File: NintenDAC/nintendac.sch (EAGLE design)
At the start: 36 parts, among them IC2 REG1117, U1 STM32F10XRXT6, X1 USB-MICROB

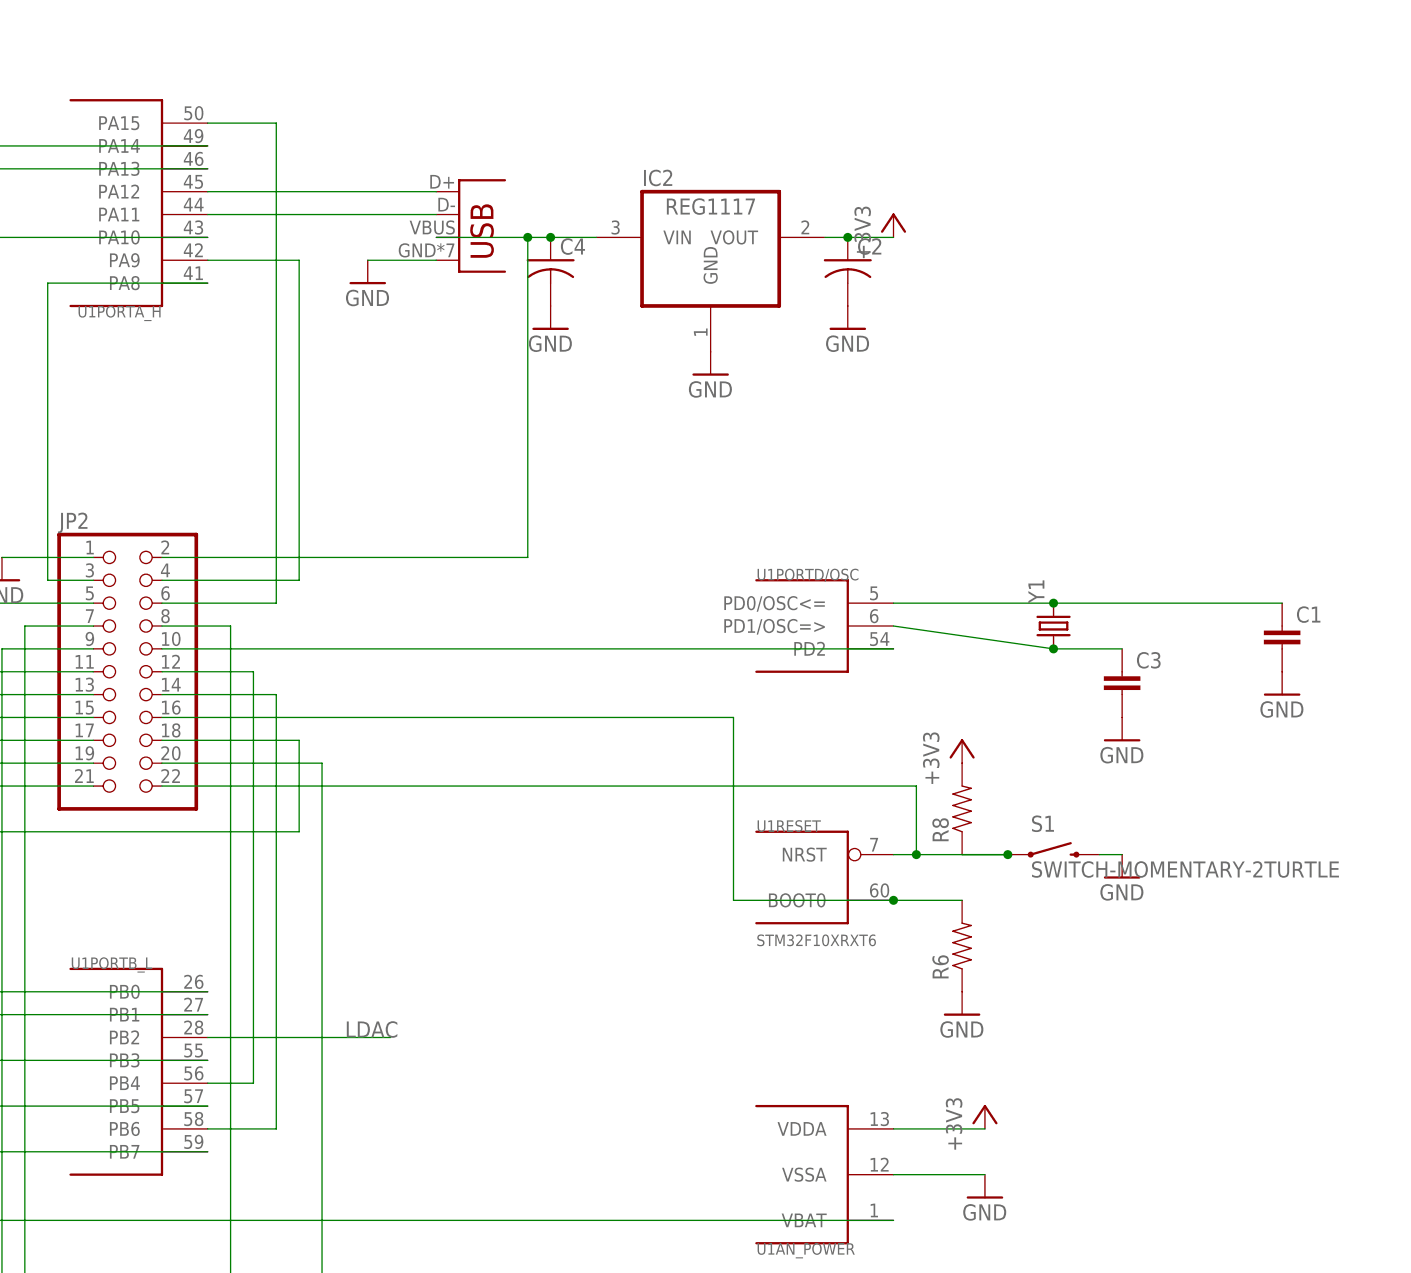
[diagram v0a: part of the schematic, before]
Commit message: board cleanup
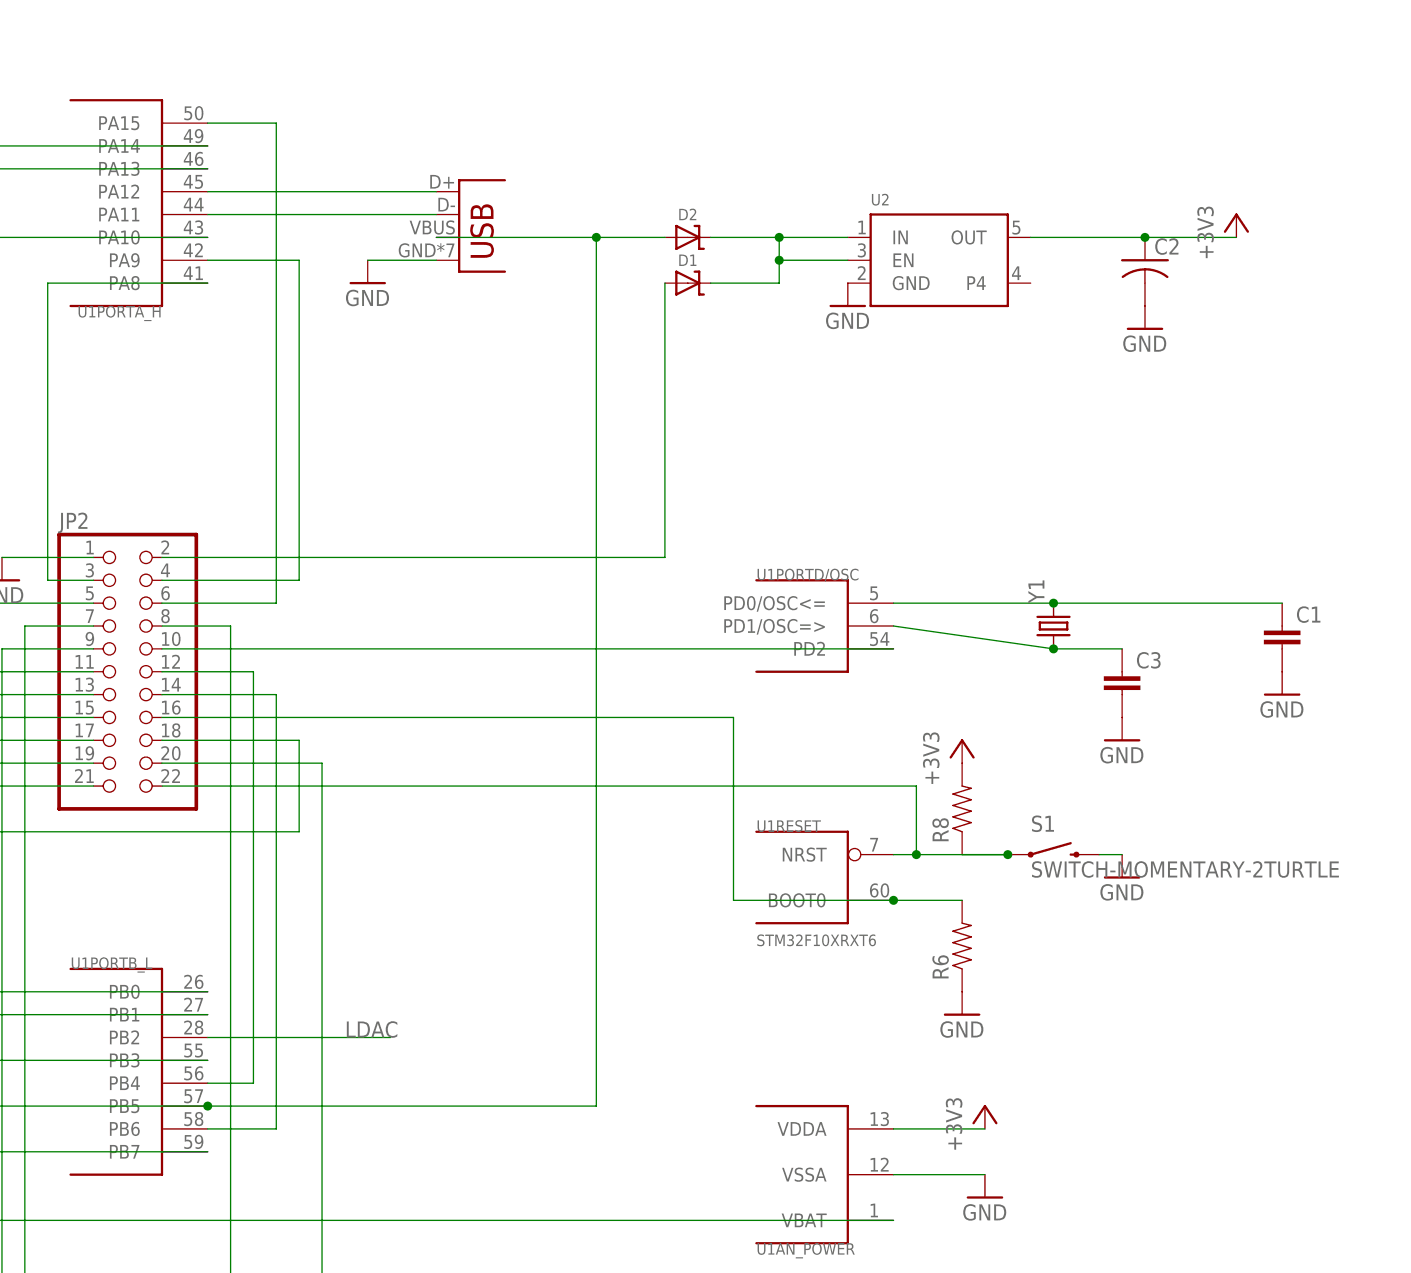
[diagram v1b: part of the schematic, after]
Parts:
- removed C4: (no value), backplane:C-USC1210
- removed IC2: REG1117, backplane:REG1117
- added D1, D2: (no value), nintendac_mini:DIODE-SCHOTTKYSOD-123
- added U2: (no value), nintendac_mini:VREG_SOT23-5
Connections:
- new net N$2: D1.C, D2.C, U2.EN, U2.IN
- net +3V3: now also U2.OUT; no longer IC2.VOUT
- net GND: now also U2.GND; no longer C4.2, IC2.GND
- net N$58: now also D2.A, X1.VBUS
- net N$66: now also D1.A; no longer C4.1, IC2.VIN, X1.VBUS
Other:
- moved on the sheet: C2
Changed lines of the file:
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@@
 <part name="GND1" library="backplane" deviceset="GND" device=""/>
 <part name="R1" library="SparkFun-Passives" deviceset="RESISTOR" device="0805-RES"/>
-<part name="IC2" library="backplane" deviceset="REG1117" device=""/>
 <part name="X1" library="backplane" deviceset="USB" device="-MICROB"/>
 <part name="GND2" library="backplane" deviceset="GND" device=""/>
@@
 <part name="+3V2" library="backplane" deviceset="+3V3" device=""/>
 <part name="GND5" library="backplane" deviceset="GND" device=""/>
-<part name="GND6" library="backplane" deviceset="GND" device=""/>
 <part name="+3V3" library="backplane" deviceset="+3V3" device=""/>
 <part name="S1" library="Adafruit Feather M0 Adalogger" deviceset="SWITCH-MOMENTARY-2" device="TURTLE"/>
@@
 <part name="GND7" library="backplane" deviceset="GND" device=""/>
 <part name="GND8" library="backplane" deviceset="GND" device=""/>
-<part name="C4" library="backplane" deviceset="C-US" device="C1210"/>
-<part name="GND9" library="backplane" deviceset="GND" device=""/>
 <part name="GND10" library="backplane" deviceset="GND" device=""/>
 <part name="GND11" library="backplane" deviceset="GND" device=""/>
@@
 <part name="GND22" library="backplane" deviceset="GND" device=""/>
 <part name="S2" library="Adafruit Feather M0 Adalogger" deviceset="SWITCH-MOMENTARY-2" device="TURTLE"/>
+<part name="D1" library="nintendac_mini" deviceset="DIODE-SCHOTTKY" device="SOD-123"/>
+<part name="D2" library="nintendac_mini" deviceset="DIODE-SCHOTTKY" device="SOD-123"/>
+<part name="U2" library="nintendac_mini" deviceset="VREG_SOT23-5" device=""/>
+<part name="GND6" library="backplane" deviceset="GND" device=""/>
 </parts>
 <sheets>
@@
 <instance part="+3V1" gate="G$1" x="-93.98" y="162.56"/>
 <instance part="C1" gate="G$1" x="190.5" y="-83.82"/>
-<instance part="C2" gate="G$1" x="142.24" y="-40.64"/>
+<instance part="C2" gate="G$1" x="175.26" y="-40.64"/>
 <instance part="Y1" gate="G$1" x="165.1" y="-81.28" rot="R90"/>
 <instance part="GND1" gate="1" x="-7.62" y="43.18"/>
 <instance part="R1" gate="G$1" x="-91.44" y="0" rot="R90"/>
-<instance part="IC2" gate="G$1" x="127" y="-38.1"/>
 <instance part="X1" gate="G$1" x="99.06" y="-40.64"/>
 <instance part="GND2" gate="1" x="172.72" y="-109.22"/>
@@
 <instance part="+3V2" gate="G$1" x="157.48" y="-134.62"/>
 <instance part="GND5" gate="1" x="88.9" y="-43.18"/>
-<instance part="GND6" gate="1" x="127" y="-53.34"/>
-<instance part="+3V3" gate="G$1" x="147.32" y="-35.56"/>
+<instance part="+3V3" gate="G$1" x="185.42" y="-35.56"/>
 <instance part="S1" gate="G$1" x="165.1" y="-106.68"/>
 <instance part="JP2" gate="A" x="60.96" y="-86.36"/>
@@
 <instance part="GND7" gate="1" x="172.72" y="-93.98"/>
 <instance part="GND8" gate="1" x="190.5" y="-88.9"/>
-<instance part="C4" gate="G$1" x="109.22" y="-40.64"/>
-<instance part="GND9" gate="1" x="109.22" y="-48.26"/>
-<instance part="GND10" gate="1" x="142.24" y="-48.26"/>
+<instance part="GND10" gate="1" x="175.26" y="-48.26"/>
 <instance part="GND11" gate="1" x="-157.48" y="-30.48"/>
 <instance part="+3V4" gate="G$1" x="-124.46" y="-35.56"/>
@@
 <instance part="GND22" gate="1" x="-180.34" y="-177.8"/>
 <instance part="S2" gate="G$1" x="-175.26" y="-175.26"/>
+<instance part="D1" gate="G$1" x="124.46" y="-43.18"/>
+<instance part="D2" gate="G$1" x="124.46" y="-38.1"/>
+<instance part="U2" gate="G$1" x="152.4" y="-40.64"/>
+<instance part="GND6" gate="1" x="142.24" y="-45.72"/>
 </instances>
 <busses>
@@
 </segment>
 <segment>
-<pinref part="IC2" gate="G$1" pin="GND"/>
-<pinref part="GND6" gate="1" pin="GND"/>
-</segment>
-<segment>
 <pinref part="GND2" gate="1" pin="GND"/>
 <pinref part="S1" gate="G$1" pin="2"/>
@@
 <pinref part="C1" gate="G$1" pin="2"/>
 <pinref part="GND8" gate="1" pin="GND"/>
-</segment>
-<segment>
-<pinref part="C4" gate="G$1" pin="2"/>
-<pinref part="GND9" gate="1" pin="GND"/>
 </segment>
 <segment>
@@
 <pinref part="GND22" gate="1" pin="GND"/>
 </segment>
+<segment>
+<pinref part="U2" gate="G$1" pin="GND"/>
+<pinref part="GND6" gate="1" pin="GND"/>
+</segment>
 </net>
 <net name="+3V3" class="0">
@@
 </segment>
 <segment>
-<pinref part="IC2" gate="G$1" pin="VOUT"/>
 <pinref part="+3V3" gate="G$1" pin="+3V3"/>
-<wire x1="147.32" y1="-38.1" x2="142.24" y2="-38.1" width="0.1524" layer="91"/>
+<wire x1="185.42" y1="-38.1" x2="175.26" y2="-38.1" width="0.1524" layer="91"/>
 <pinref part="C2" gate="G$1" pin="1"/>
-<wire x1="142.24" y1="-38.1" x2="139.7" y2="-38.1" width="0.1524" layer="91"/>
-<junction x="142.24" y="-38.1"/>
+<pinref part="U2" gate="G$1" pin="OUT"/>
+<wire x1="162.56" y1="-38.1" x2="175.26" y2="-38.1" width="0.1524" layer="91"/>
+<junction x="175.26" y="-38.1"/>
 </segment>
 <segment>
@@
 <pinref part="JP2" gate="A" pin="13"/>
 <wire x1="43.18" y1="-88.9" x2="58.42" y2="-88.9" width="0.1524" layer="91"/>
+<pinref part="D2" gate="G$1" pin="A"/>
+<pinref part="X1" gate="G$1" pin="VBUS"/>
+<wire x1="96.52" y1="-38.1" x2="114.3" y2="-38.1" width="0.1524" layer="91"/>
+<wire x1="114.3" y1="-38.1" x2="121.92" y2="-38.1" width="0.1524" layer="91"/>
+<wire x1="71.12" y1="-134.62" x2="114.3" y2="-134.62" width="0.1524" layer="91"/>
+<wire x1="114.3" y1="-134.62" x2="114.3" y2="-38.1" width="0.1524" layer="91"/>
+<junction x="71.12" y="-134.62"/>
+<junction x="114.3" y="-38.1"/>
 </segment>
 </net>
@@
 </segment>
 </net>
+<net name="N$2" class="0">
+<segment>
+<pinref part="D2" gate="G$1" pin="C"/>
+<pinref part="U2" gate="G$1" pin="IN"/>
+<wire x1="127" y1="-38.1" x2="134.62" y2="-38.1" width="0.1524" layer="91"/>
+<pinref part="D1" gate="G$1" pin="C"/>
+<wire x1="134.62" y1="-38.1" x2="142.24" y2="-38.1" width="0.1524" layer="91"/>
+<wire x1="127" y1="-43.18" x2="134.62" y2="-43.18" width="0.1524" layer="91"/>
+<wire x1="134.62" y1="-43.18" x2="134.62" y2="-40.64" width="0.1524" layer="91"/>
+<junction x="134.62" y="-38.1"/>
+<pinref part="U2" gate="G$1" pin="EN"/>
+<wire x1="134.62" y1="-40.64" x2="134.62" y2="-38.1" width="0.1524" layer="91"/>
+<wire x1="142.24" y1="-40.64" x2="134.62" y2="-40.64" width="0.1524" layer="91"/>
+<junction x="134.62" y="-40.64"/>
+</segment>
+</net>
 <net name="N$66" class="0">
 <segment>
 <pinref part="JP2" gate="A" pin="2"/>
-<pinref part="X1" gate="G$1" pin="VBUS"/>
-<pinref part="IC2" gate="G$1" pin="VIN"/>
-<wire x1="96.52" y1="-38.1" x2="106.68" y2="-38.1" width="0.1524" layer="91"/>
-<pinref part="C4" gate="G$1" pin="1"/>
-<wire x1="106.68" y1="-38.1" x2="109.22" y2="-38.1" width="0.1524" layer="91"/>
-<wire x1="109.22" y1="-38.1" x2="114.3" y2="-38.1" width="0.1524" layer="91"/>
-<junction x="109.22" y="-38.1"/>
-<wire x1="66.04" y1="-73.66" x2="106.68" y2="-73.66" width="0.1524" layer="91"/>
-<wire x1="106.68" y1="-73.66" x2="106.68" y2="-38.1" width="0.1524" layer="91"/>
-<junction x="106.68" y="-38.1"/>
-</segment>
-</net>
+<pinref part="D1" gate="G$1" pin="A"/>
+<wire x1="66.04" y1="-73.66" x2="121.92" y2="-73.66" width="0.1524" layer="91"/>
+<wire x1="121.92" y1="-73.66" x2="121.92" y2="-43.18" width="0.1524" layer="91"/>
+</segment>
+</net>
